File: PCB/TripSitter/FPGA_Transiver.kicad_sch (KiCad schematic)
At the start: 1 part, among them U1 XC7A100T-FGG484

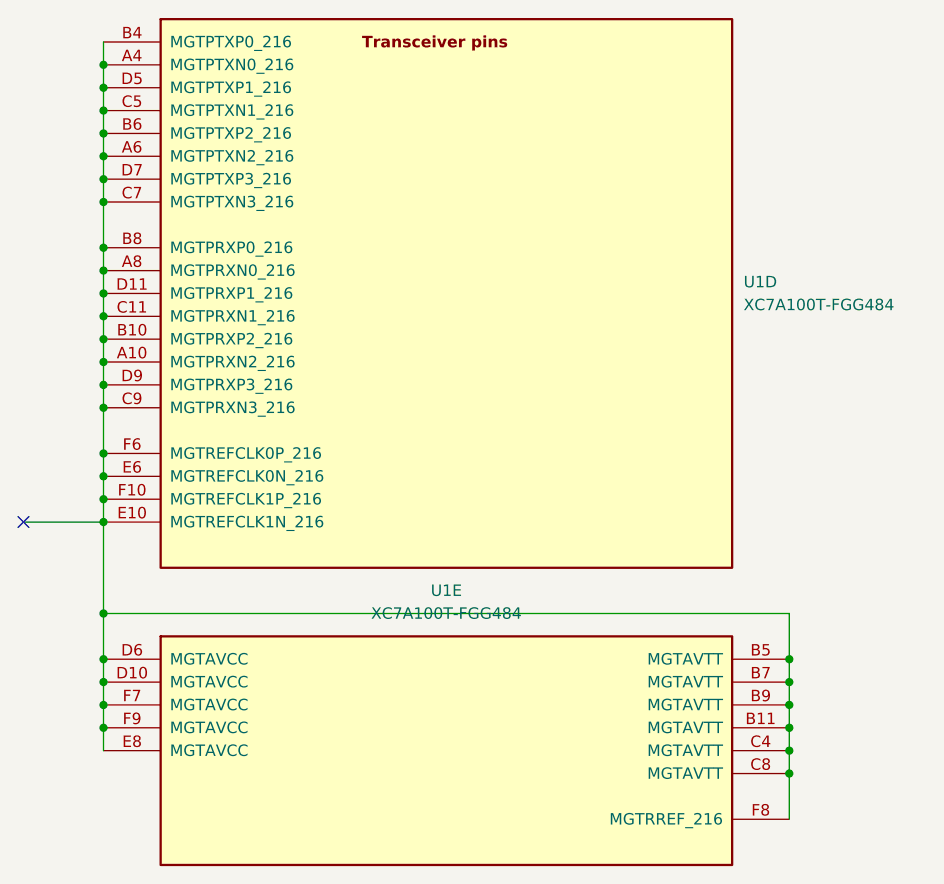
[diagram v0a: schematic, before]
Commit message: attempt at routing
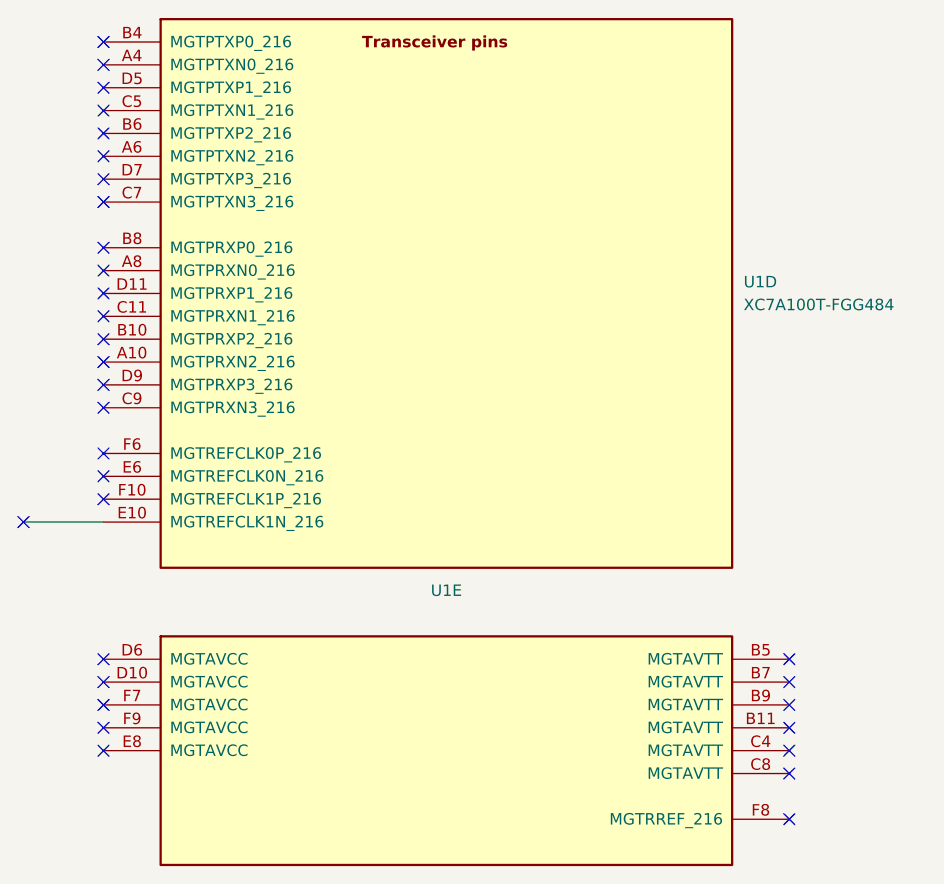
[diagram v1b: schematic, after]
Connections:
- now unconnected: U1.A10 (MGTPRXN2_216), U1.A4 (MGTPTXN0_216), U1.A6 (MGTPTXN2_216), U1.A8 (MGTPRXN0_216), U1.B10 (MGTPRXP2_216), U1.B11 (MGTAVTT), U1.B4 (MGTPTXP0_216), U1.B5 (MGTAVTT), U1.B6 (MGTPTXP2_216), U1.B7 (MGTAVTT), U1.B8 (MGTPRXP0_216), U1.B9 (MGTAVTT), U1.C11 (MGTPRXN1_216), U1.C4 (MGTAVTT), U1.C5 (MGTPTXN1_216), U1.C7 (MGTPTXN3_216), U1.C8 (MGTAVTT), U1.C9 (MGTPRXN3_216), U1.D10 (MGTAVCC), U1.D11 (MGTPRXP1_216), U1.D5 (MGTPTXP1_216), U1.D6 (MGTAVCC), U1.D7 (MGTPTXP3_216), U1.D9 (MGTPRXP3_216), U1.E10 (MGTREFCLK1N_216), U1.E6 (MGTREFCLK0N_216), U1.E8 (MGTAVCC), U1.F10 (MGTREFCLK1P_216), U1.F6 (MGTREFCLK0P_216), U1.F7 (MGTAVCC), U1.F8 (MGTRREF_216), U1.F9 (MGTAVCC)
- no-connect marks 1 -> 32
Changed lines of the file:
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@@
     (company "NTNU x Nordic Semiconductor")
   )
-  (junction (at 50.8 54.61) (diameter 0) (color 0 0 0 0)
-  )
-  (junction (at 50.8 115.57) (diameter 0) (color 0 0 0 0)
-  )
-  (junction (at 50.8 80.01) (diameter 0) (color 0 0 0 0)
-  )
-  (junction (at 50.8 49.53) (diameter 0) (color 0 0 0 0)
-  )
-  (junction (at 127 123.19) (diameter 0) (color 0 0 0 0)
-  )
-  (junction (at 50.8 95.25) (diameter 0) (color 0 0 0 0)
-  )
-  (junction (at 50.8 90.17) (diameter 0) (color 0 0 0 0)
-  )
-  (junction (at 50.8 82.55) (diameter 0) (color 0 0 0 0)
-  )
-  (junction (at 50.8 57.15) (diameter 0) (color 0 0 0 0)
-  )
-  (junction (at 50.8 64.77) (diameter 0) (color 0 0 0 0)
-  )
-  (junction (at 50.8 59.69) (diameter 0) (color 0 0 0 0)
-  )
-  (junction (at 50.8 87.63) (diameter 0) (color 0 0 0 0)
-  )
-  (junction (at 50.8 77.47) (diameter 0) (color 0 0 0 0)
-  )
-  (junction (at 50.8 52.07) (diameter 0) (color 0 0 0 0)
-  )
-  (junction (at 50.8 69.85) (diameter 0) (color 0 0 0 0)
-  )
-  (junction (at 127 120.65) (diameter 0) (color 0 0 0 0)
-  )
-  (junction (at 50.8 92.71) (diameter 0) (color 0 0 0 0)
-  )
-  (junction (at 50.8 72.39) (diameter 0) (color 0 0 0 0)
-  )
-  (junction (at 50.8 105.41) (diameter 0) (color 0 0 0 0)
-  )
-  (junction (at 50.8 118.11) (diameter 0) (color 0 0 0 0)
-  )
-  (junction (at 50.8 44.45) (diameter 0) (color 0 0 0 0)
-  )
-  (junction (at 50.8 67.31) (diameter 0) (color 0 0 0 0)
-  )
-  (junction (at 127 113.03) (diameter 0) (color 0 0 0 0)
-  )
-  (junction (at 50.8 46.99) (diameter 0) (color 0 0 0 0)
-  )
-  (junction (at 50.8 113.03) (diameter 0) (color 0 0 0 0)
-  )
-  (junction (at 50.8 110.49) (diameter 0) (color 0 0 0 0)
-  )
-  (junction (at 127 115.57) (diameter 0) (color 0 0 0 0)
-  )
-  (junction (at 127 110.49) (diameter 0) (color 0 0 0 0)
-  )
-  (junction (at 50.8 74.93) (diameter 0) (color 0 0 0 0)
-  )
-  (junction (at 127 118.11) (diameter 0) (color 0 0 0 0)
-  )
+  (no_connect (at 50.8 67.31))
+  (no_connect (at 50.8 64.77))
+  (no_connect (at 50.8 54.61))
+  (no_connect (at 50.8 57.15))
+  (no_connect (at 50.8 118.11))
+  (no_connect (at 50.8 44.45))
   (no_connect (at 41.91 95.25))
-  (wire (pts (xy 50.8 64.77) (xy 50.8 67.31))
-    (stroke (width 0) (type default))
-  )
-  (wire (pts (xy 50.8 41.91) (xy 50.8 44.45))
-    (stroke (width 0) (type default))
-  )
-  (wire (pts (xy 127 115.57) (xy 127 118.11))
-    (stroke (width 0) (type default))
-  )
-  (wire (pts (xy 50.8 67.31) (xy 50.8 69.85))
-    (stroke (width 0) (type default))
-  )
-  (wire (pts (xy 50.8 95.25) (xy 50.8 105.41))
-    (stroke (width 0) (type default))
-  )
-  (wire (pts (xy 127 123.19) (xy 127 128.27))
-    (stroke (width 0) (type default))
-  )
-  (wire (pts (xy 50.8 72.39) (xy 50.8 74.93))
-    (stroke (width 0) (type default))
-  )
-  (wire (pts (xy 50.8 87.63) (xy 50.8 90.17))
-    (stroke (width 0) (type default))
-  )
-  (wire (pts (xy 127 110.49) (xy 127 105.41))
-    (stroke (width 0) (type default))
-  )
-  (wire (pts (xy 50.8 90.17) (xy 50.8 92.71))
-    (stroke (width 0) (type default))
-  )
-  (wire (pts (xy 50.8 77.47) (xy 50.8 80.01))
-    (stroke (width 0) (type default))
-  )
-  (wire (pts (xy 50.8 110.49) (xy 50.8 113.03))
-    (stroke (width 0) (type default))
-  )
-  (wire (pts (xy 50.8 52.07) (xy 50.8 54.61))
-    (stroke (width 0) (type default))
-  )
-  (wire (pts (xy 50.8 115.57) (xy 50.8 118.11))
-    (stroke (width 0) (type default))
-  )
-  (wire (pts (xy 50.8 105.41) (xy 127 105.41))
-    (stroke (width 0) (type default))
-  )
-  (wire (pts (xy 127 113.03) (xy 127 115.57))
-    (stroke (width 0) (type default))
-  )
-  (wire (pts (xy 50.8 49.53) (xy 50.8 52.07))
-    (stroke (width 0) (type default))
-  )
-  (wire (pts (xy 50.8 74.93) (xy 50.8 77.47))
-    (stroke (width 0) (type default))
-  )
-  (wire (pts (xy 127 118.11) (xy 127 120.65))
-    (stroke (width 0) (type default))
-  )
-  (wire (pts (xy 50.8 59.69) (xy 50.8 64.77))
-    (stroke (width 0) (type default))
-  )
-  (wire (pts (xy 50.8 54.61) (xy 50.8 57.15))
-    (stroke (width 0) (type default))
-  )
-  (wire (pts (xy 50.8 105.41) (xy 50.8 110.49))
-    (stroke (width 0) (type default))
-  )
-  (wire (pts (xy 50.8 80.01) (xy 50.8 82.55))
-    (stroke (width 0) (type default))
-  )
-  (wire (pts (xy 50.8 44.45) (xy 50.8 46.99))
-    (stroke (width 0) (type default))
-  )
-  (wire (pts (xy 50.8 118.11) (xy 50.8 120.65))
-    (stroke (width 0) (type default))
-  )
-  (wire (pts (xy 50.8 69.85) (xy 50.8 72.39))
-    (stroke (width 0) (type default))
-  )
+  (no_connect (at 50.8 115.57))
+  (no_connect (at 50.8 52.07))
+  (no_connect (at 50.8 59.69))
+  (no_connect (at 50.8 80.01))
+  (no_connect (at 127 110.49))
+  (no_connect (at 50.8 72.39))
+  (no_connect (at 50.8 46.99))
+  (no_connect (at 50.8 120.65))
+  (no_connect (at 50.8 77.47))
+  (no_connect (at 50.8 113.03))
+  (no_connect (at 50.8 92.71))
+  (no_connect (at 127 123.19))
+  (no_connect (at 50.8 41.91))
+  (no_connect (at 50.8 90.17))
+  (no_connect (at 50.8 74.93))
+  (no_connect (at 50.8 69.85))
+  (no_connect (at 127 120.65))
+  (no_connect (at 50.8 82.55))
+  (no_connect (at 127 115.57))
+  (no_connect (at 50.8 110.49))
+  (no_connect (at 127 128.27))
+  (no_connect (at 50.8 49.53))
+  (no_connect (at 127 118.11))
+  (no_connect (at 50.8 87.63))
+  (no_connect (at 127 113.03))
   (wire (pts (xy 41.91 95.25) (xy 50.8 95.25))
-    (stroke (width 0) (type default))
-  )
-  (wire (pts (xy 127 110.49) (xy 127 113.03))
-    (stroke (width 0) (type default))
-  )
-  (wire (pts (xy 50.8 46.99) (xy 50.8 49.53))
-    (stroke (width 0) (type default))
-  )
-  (wire (pts (xy 50.8 92.71) (xy 50.8 95.25))
-    (stroke (width 0) (type default))
-  )
-  (wire (pts (xy 50.8 57.15) (xy 50.8 59.69))
-    (stroke (width 0) (type default))
-  )
-  (wire (pts (xy 127 120.65) (xy 127 123.19))
-    (stroke (width 0) (type default))
-  )
-  (wire (pts (xy 50.8 113.03) (xy 50.8 115.57))
-    (stroke (width 0) (type default))
-  )
-  (wire (pts (xy 50.8 82.55) (xy 50.8 87.63))
     (stroke (width 0) (type default))
   )
@@
     )
     (property "Value" "XC7A100T-FGG484" (at 88.9 105.41 0)
-      (effects (font (size 1.27 1.27)))
+      (effects (font (size 1.27 1.27)) hide)
     )
     (property "Footprint" "Package_BGA:Xilinx_FGG484" (at 88.9 113.03 0)
